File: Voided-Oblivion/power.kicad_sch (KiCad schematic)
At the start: 133 parts, among them Q1 AO3401, Q10 BC847B, Q11 BC847B, Q13 NCE4009S, Q14 NCE4009S, Q2 AO4407A, Q3 BC857, Q4 AO4407A, Q5 AO4407A, Q6 AO4407A, Q7 AO4407A, Q8 BC847B, Q9 BC847B, U10 TLV431BQDBZR, U11 LM2903, U12 AP2171WG-7, U13 TPD2E2U06DRL, U14 TPD2E2U06DRL, U15 LM66100DCKT, U16 AP2171WG-7, U17 LM74700QDDF, U18 LM74700QDDF, U2 TS3USB30ERSWR, U5 TPS54302, U6 TPS54302, U7 TLV76733DRVR, U9 LM66100DCKT

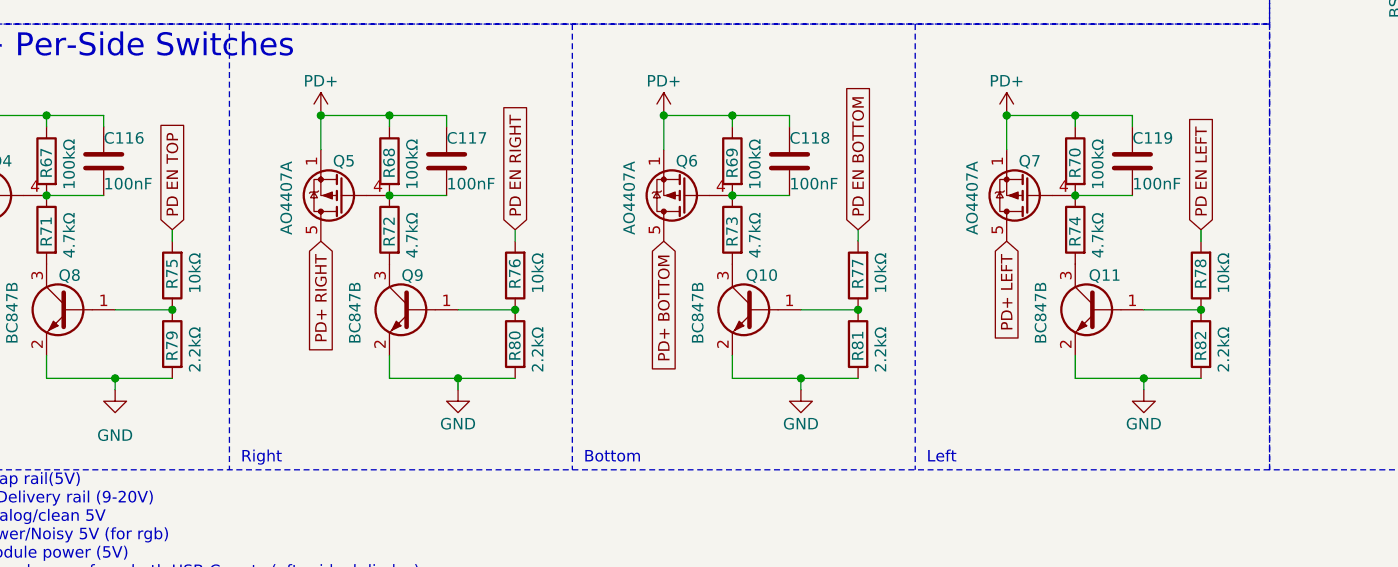
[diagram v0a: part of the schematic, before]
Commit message: BOMB update  (ignore the "B" on the end of that first word, it has no significant meaning) and some library linking
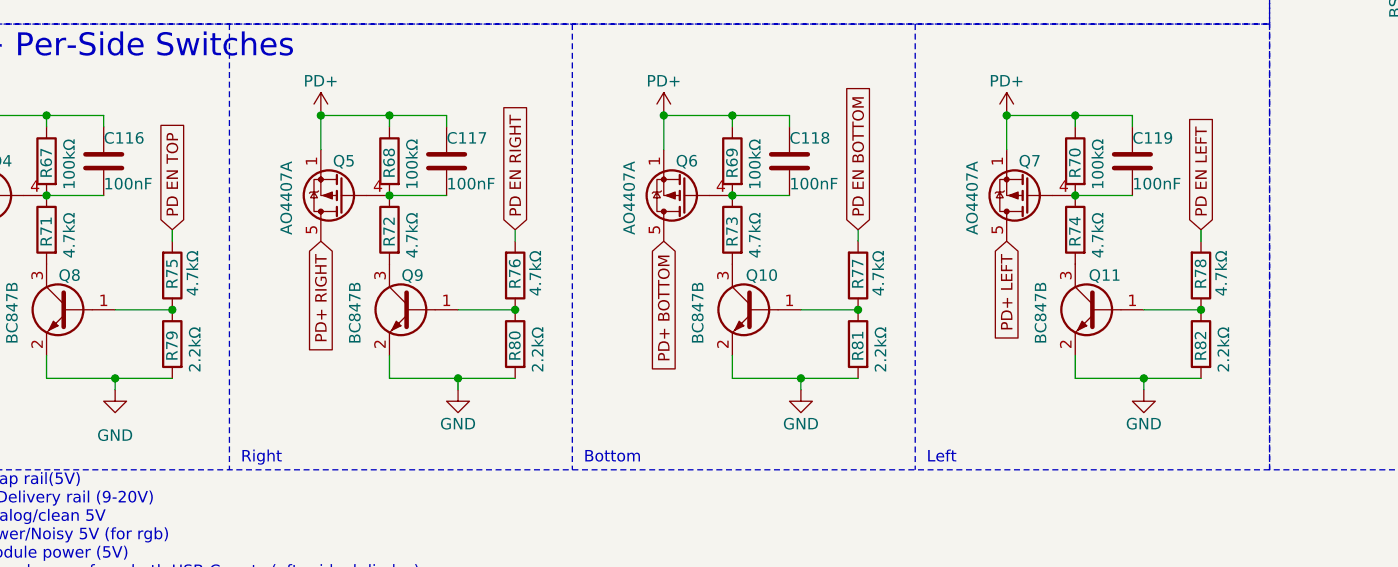
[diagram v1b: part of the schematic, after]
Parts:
- C121, C40, C77: LCSC C315248 -> C89632; MPN CL05A106MP5NUNC -> CL31B106KBHNNNE
- C26, C31: LCSC (none) -> C89632; MPN (none) -> CL31B106KBHNNNE; Manufacturer (none) -> Samsung Electro-Mechanics
- C28, C29, C34, C35: LCSC (none) -> C12891; MPN (none) -> CL31A226KAHNNNE; Manufacturer (none) -> Samsung Electro-Mechanics
- Q13, Q14: MPN (none) -> NCE4009S; Manufacturer (none) -> Wuxi NCE Power Semiconductor
- R22: MPN (none) -> 0402WGF5101TCE; Manufacturer (none) -> UNI-ROYAL(Uniroyal Elec)
- R31: Manufacturer (none) -> Viking Tech
- R75, R76, R77, R78: value 10kΩ -> 4.7kΩ; LCSC C25744 -> C25900; MPN 0402WGF1002TCE -> 0402WGF4701TCE
- R79, R80, R81, R82: LCSC (none) -> C25879; MPN (none) -> 0402WGF2201TCE; Manufacturer (none) -> UNI-ROYAL(Uniroyal Elec)
- U10: MPN (none) -> TLV431BQDBZR; Manufacturer (none) -> Texas Instruments
- U17, U18: MPN (none) -> LM74700QDDFRQ1; Manufacturer (none) -> Texas Instruments
- USB1, USB2: MPN (none) -> HC-TYPE-C-16P-01A; Manufacturer (none) -> HCTL
